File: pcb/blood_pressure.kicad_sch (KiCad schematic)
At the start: 18 parts, among them J1 Barrel_Jack, Q1 PMOS, SW1 SW_Push, SW2 SW_SPST, U1 PicoW, U2 3073

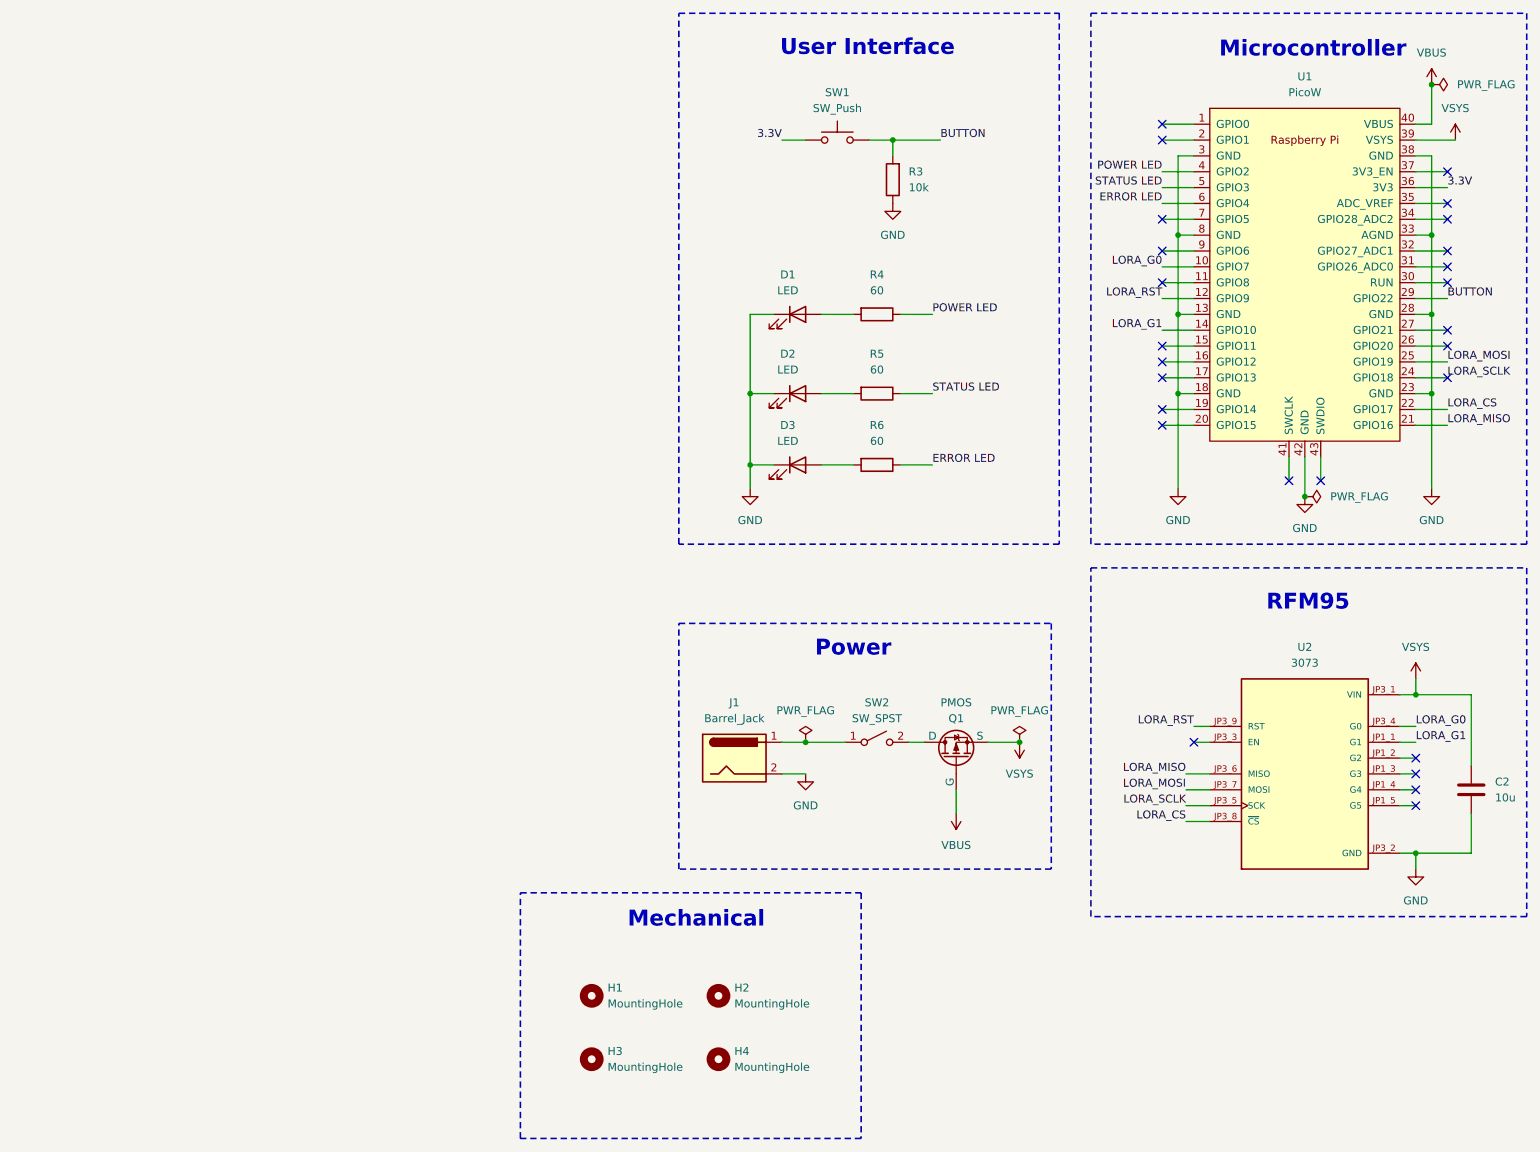
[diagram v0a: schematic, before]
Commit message: Final
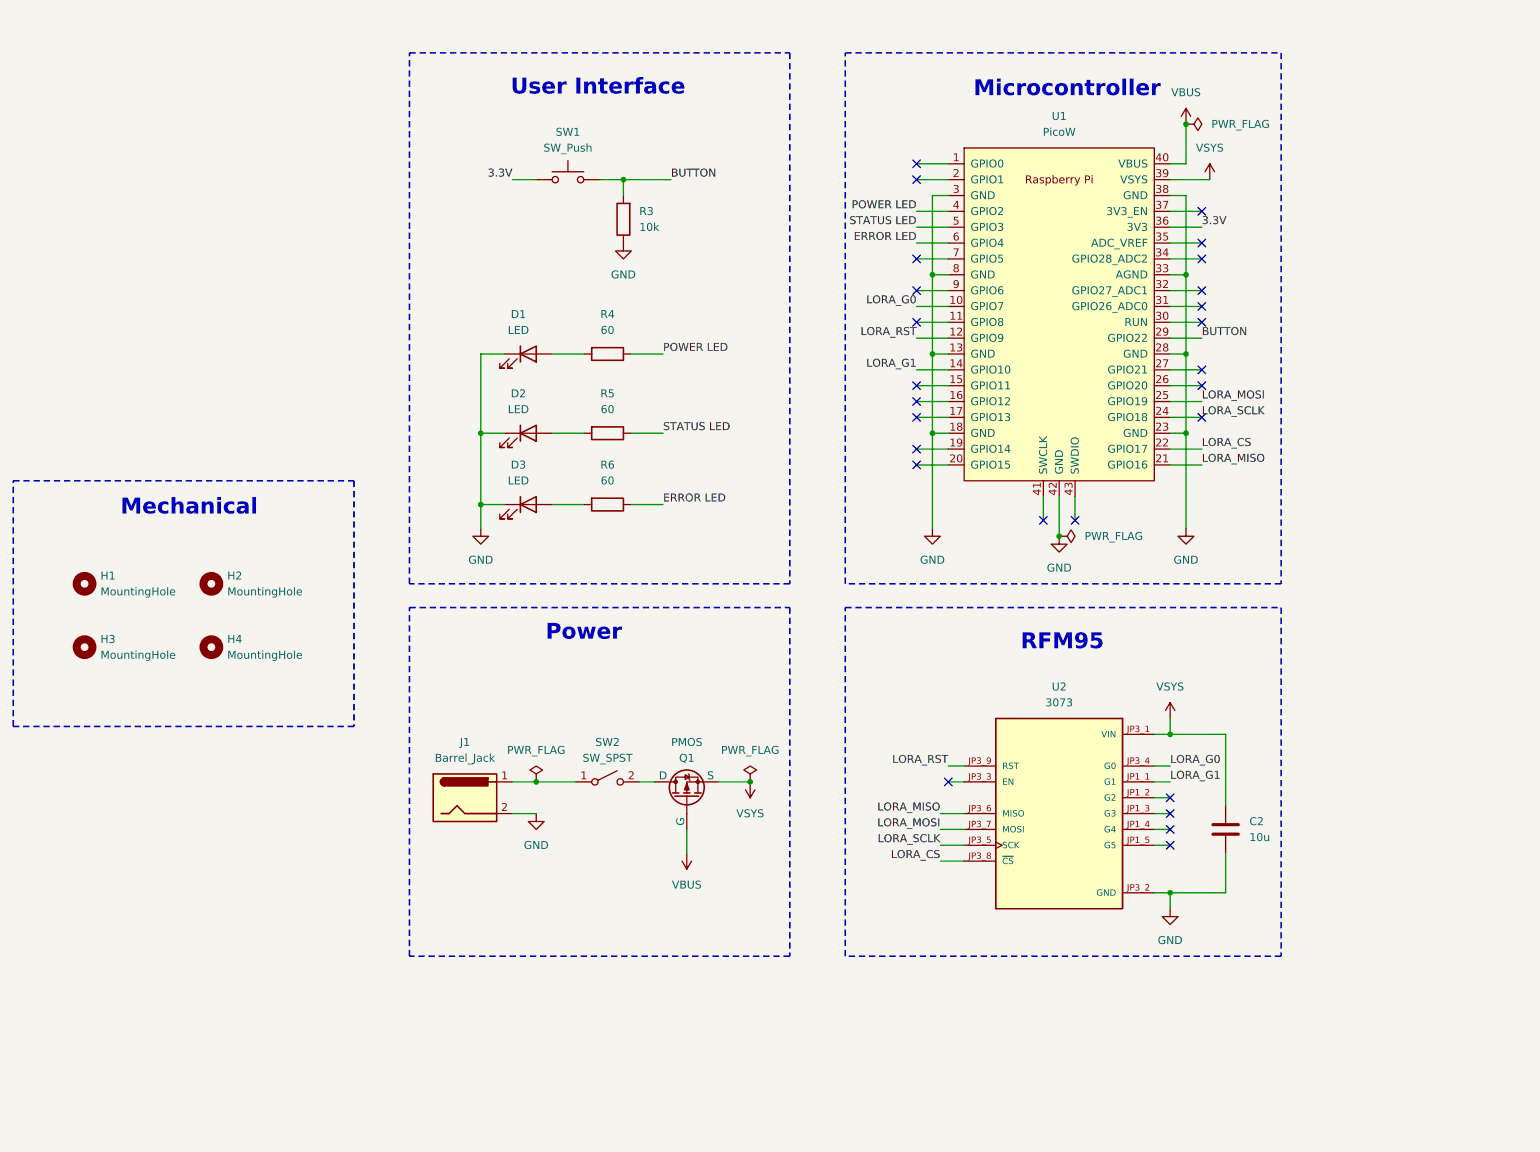
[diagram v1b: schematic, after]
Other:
- company: (none) -> Cornell University
- moved on the sheet: C2, D1, D2, D3, H1, H2, H3, H4, J1, Q1, R3, R4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
